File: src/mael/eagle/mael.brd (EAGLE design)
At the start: 99.6 x 79.1 mm, 12 parts

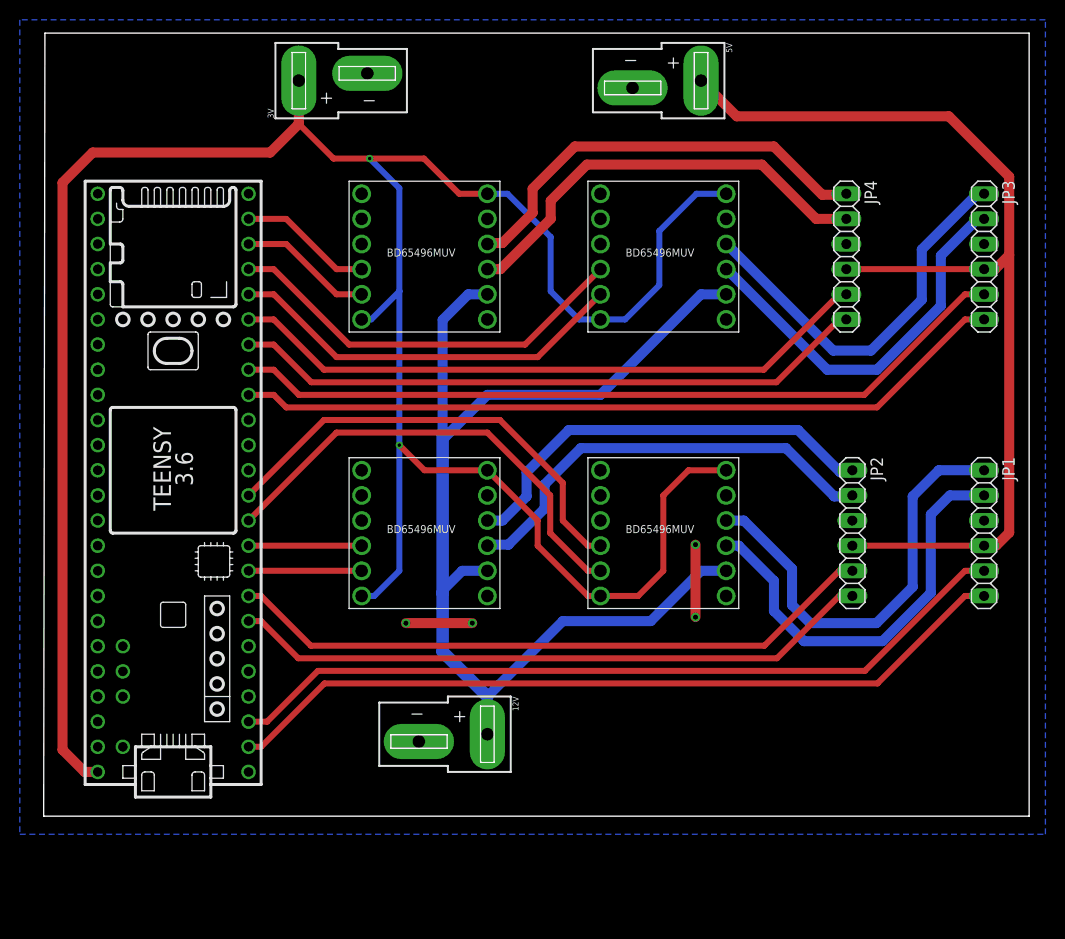
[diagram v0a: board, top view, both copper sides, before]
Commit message: Finish up mael motor PCB
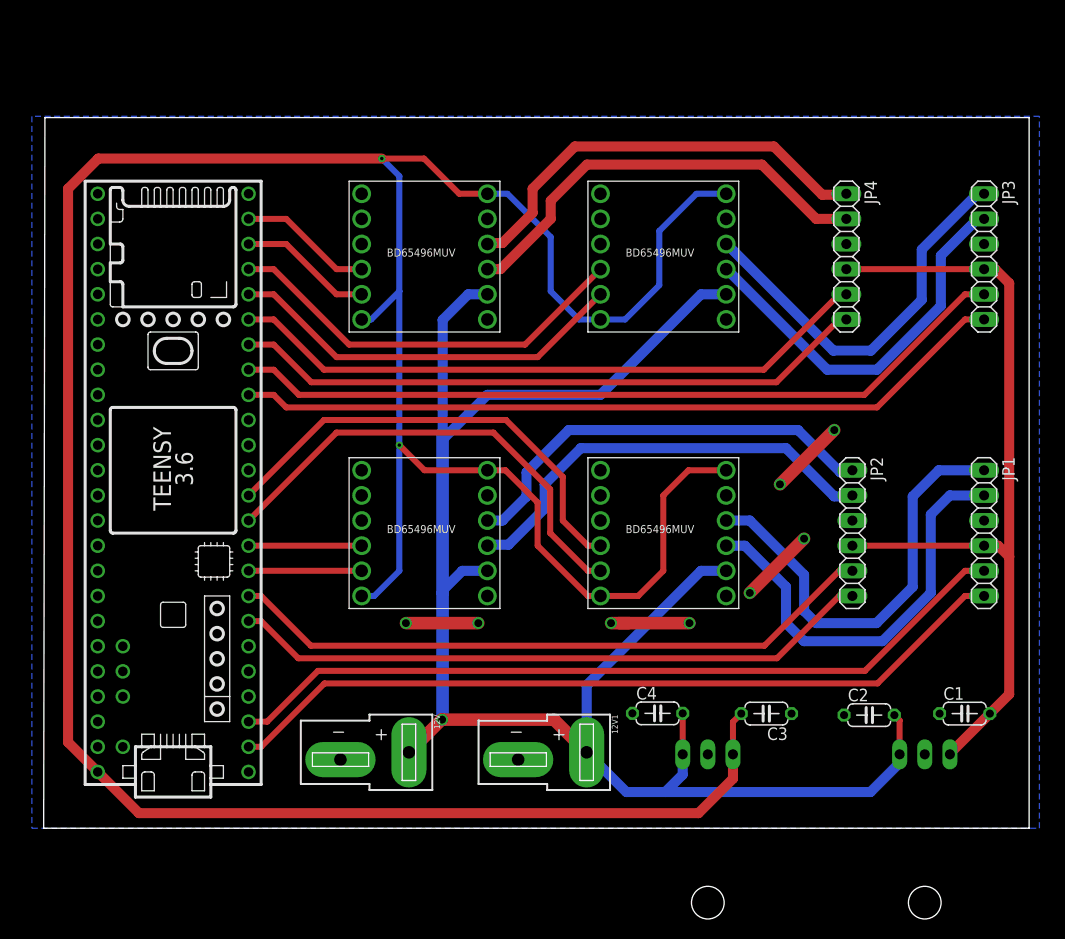
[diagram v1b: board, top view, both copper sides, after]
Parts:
- removed 3V, 5V: (no value), SparkFun-Connectors:DEANS
- added 12V1: (no value), SparkFun-Connectors:DEANS
- added C1, C2, C3, C4: (no value), rcl:C050-024X044
- added IC1, IC2: (no value), v-reg:78XXL
- moved 12V 8.13 mm to (36.9, 6.45)
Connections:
- net +12V: now also 12V1.+, C2.2, C4.2, IC1.IN, IC2.IN
- net +3V3: now also C3.2, IC1.OUT; no longer 3V.+
- net +5V: now also C1.2, IC2.OUT; no longer 5V.+
- net GND: now also 12V1.-, C1.1, C2.1, C3.1, C4.1; no longer 3V.-, 5V.-
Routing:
- net +3V3: track 261.4 -> 324.5 mm
- net +12V: track 134.9 -> 197.5 mm, vias 0 -> 1
- net +5V: track 104.6 -> 84.8 mm
- net GND: track 14.0 -> 31.8 mm, vias 4 -> 8
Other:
- board size 99.6 x 79.1 mm -> 99.6 x 71.8 mm
